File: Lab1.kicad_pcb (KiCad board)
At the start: 2 copper layers, 31 x 27 mm, 15 parts, among them J1 Conn_02x05_Counter_Clockwise, U1 STM32F407VGTx, Y1 Crystal

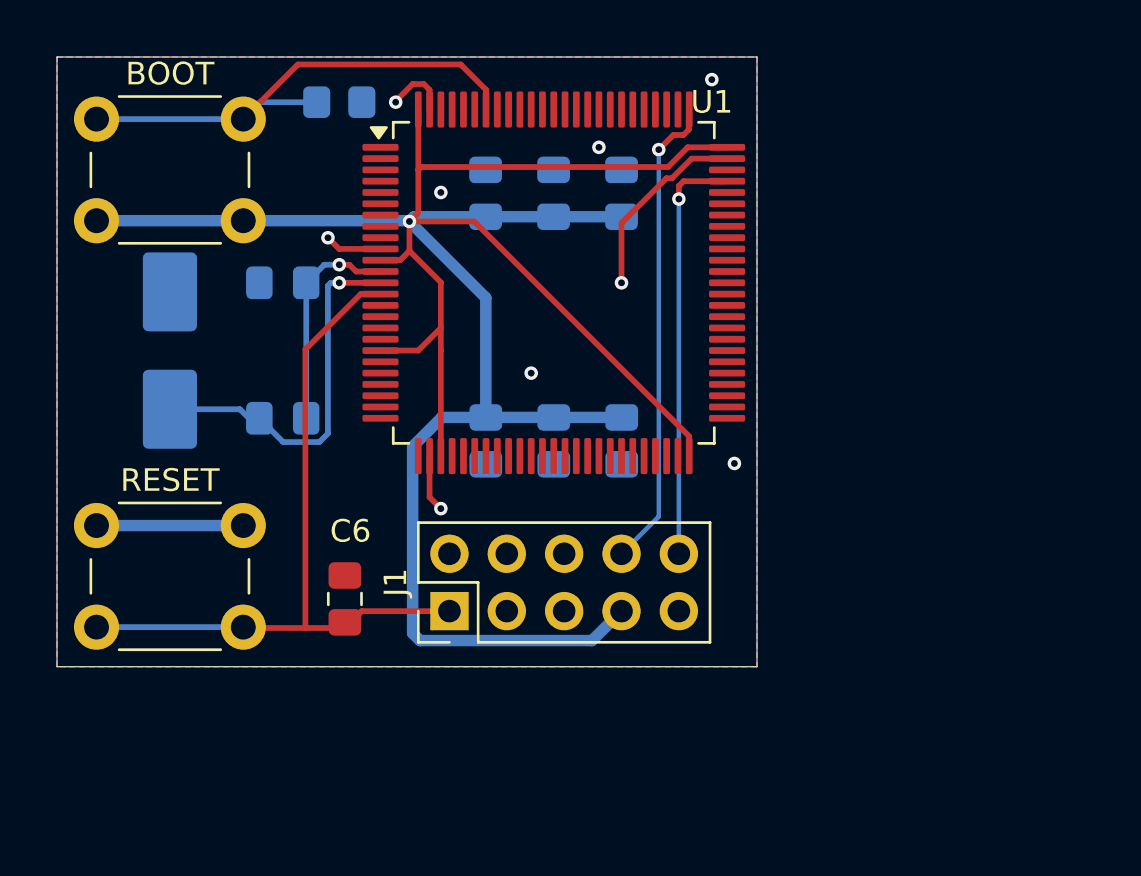
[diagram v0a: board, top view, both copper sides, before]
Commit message: feat: add tracing
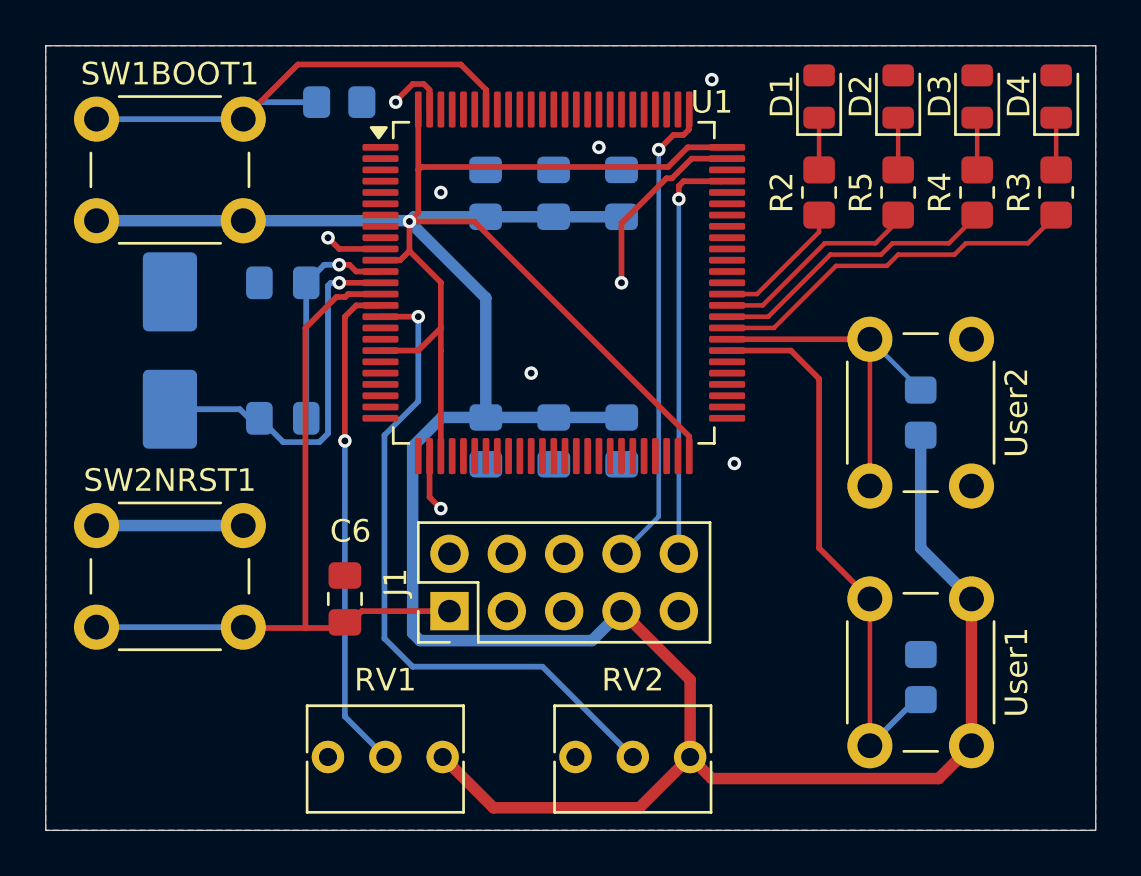
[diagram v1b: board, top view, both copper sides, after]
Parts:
- added D1: LED Blue, LED_SMD:LED_0805_2012Metric, F.Cu at (151.8, 89.8)
- added D2: LED Red, LED_SMD:LED_0805_2012Metric, F.Cu at (155.2, 89.8)
- added D3: LED Orange, LED_SMD:LED_0805_2012Metric, F.Cu at (158.8, 89.8)
- added D4: LED Green, LED_SMD:LED_0805_2012Metric, F.Cu at (162.2, 89.8)
- added R2: R 30 Ohm, Resistor_SMD:R_0805_2012Metric_Pad1.20x1.40mm_HandSolder, F.Cu at (151.8, 94.0)
- added R3: R 100 Ohm, Resistor_SMD:R_0805_2012Metric_Pad1.20x1.40mm_HandSolder, F.Cu at (162.2, 94.0)
- added R4: R 100 Ohm, Resistor_SMD:R_0805_2012Metric_Pad1.20x1.40mm_HandSolder, F.Cu at (158.8, 94.0)
- added R5: R 100 Ohm, Resistor_SMD:R_0805_2012Metric_Pad1.20x1.40mm_HandSolder, F.Cu at (155.2, 94.0)
- added R6: R 10 kOhm, Resistor_SMD:R_0805_2012Metric_Pad1.20x1.40mm_HandSolder, B.Cu at (156.3, 115.5)
- added R7: R 10 kOhm, Resistor_SMD:R_0805_2012Metric_Pad1.20x1.40mm_HandSolder, B.Cu at (156.2, 103.8)
- added RV1: 10 kOhm, Potentiometer_THT:Potentiometer_Bourns_3266Y_Vertical, F.Cu at (135.1, 119.0)
- added RV2: 10 kOhm, Potentiometer_THT:Potentiometer_Bourns_3266Y_Vertical, F.Cu at (146.0, 119.0)
- added User1: SW_Push, Button_Switch_THT:SW_PUSH_6mm, F.Cu at (158.5, 112.0)
- added User2: SW_Push, Button_Switch_THT:SW_PUSH_6mm, F.Cu at (158.5, 100.5)
- renumbered BOOT to SW1BOOT1, RESET to SW2NRST1
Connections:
- U1 pad 15: unconnected-(U1-PC0-Pad15) -> /ADC_1
- U1 pad 16: unconnected-(U1-PC1-Pad16) -> /ADC_2
- U1 pad 57: unconnected-(U1-PD10-Pad57) -> /UButton_1
- U1 pad 58: unconnected-(U1-PD11-Pad58) -> /UButton_2
- U1 pad 59: unconnected-(U1-PD12-Pad59) -> /LED_Green
- U1 pad 60: unconnected-(U1-PD13-Pad60) -> /LED_Orange
- U1 pad 61: unconnected-(U1-PD14-Pad61) -> /LED_Red
- U1 pad 62: unconnected-(U1-PD15-Pad62) -> /LED_Blue
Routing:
- net +3.3V: track 113.5 -> 162.2 mm
- net /ADC_2: track 0.00 -> 29.7 mm, vias 0 -> 1
- net /UButton_1: track 0.00 -> 24.9 mm
- net /ADC_1: track 0.00 -> 22.0 mm, vias 0 -> 1
- net /LED_Green: track 0.00 -> 16.7 mm
- net /UButton_2: track 0.00 -> 16.0 mm
- net /LED_Orange: track 0.00 -> 12.9 mm
- net /LED_Red: track 0.00 -> 9.38 mm
- net /LED_Blue: track 0.00 -> 5.96 mm
- net Net-(D4-K): track 0.00 -> 2.31 mm
- net Net-(D3-K): track 0.00 -> 2.31 mm
- net Net-(D2-K): track 0.00 -> 2.31 mm
- net Net-(D1-K): track 0.00 -> 2.31 mm
- net /NRST: track 33.7 -> 34.3 mm
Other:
- board size 31 x 27 mm -> 46.5 x 34.8 mm
